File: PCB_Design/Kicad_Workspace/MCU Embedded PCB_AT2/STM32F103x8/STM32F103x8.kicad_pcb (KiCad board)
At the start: 2 copper layers, 68.8 x 61 mm, 16 parts, among them J1 Conn_01x17, J2 Conn_01x05, J3 Conn_01x01, J4 USB_A, J5 Conn_01x04, J6 Conn_01x08, SW1 SW_Push, U1 STM32F103C8Tx, U2 AP2204R-3.3, Y1 8MHz, Y2 32.768kHz

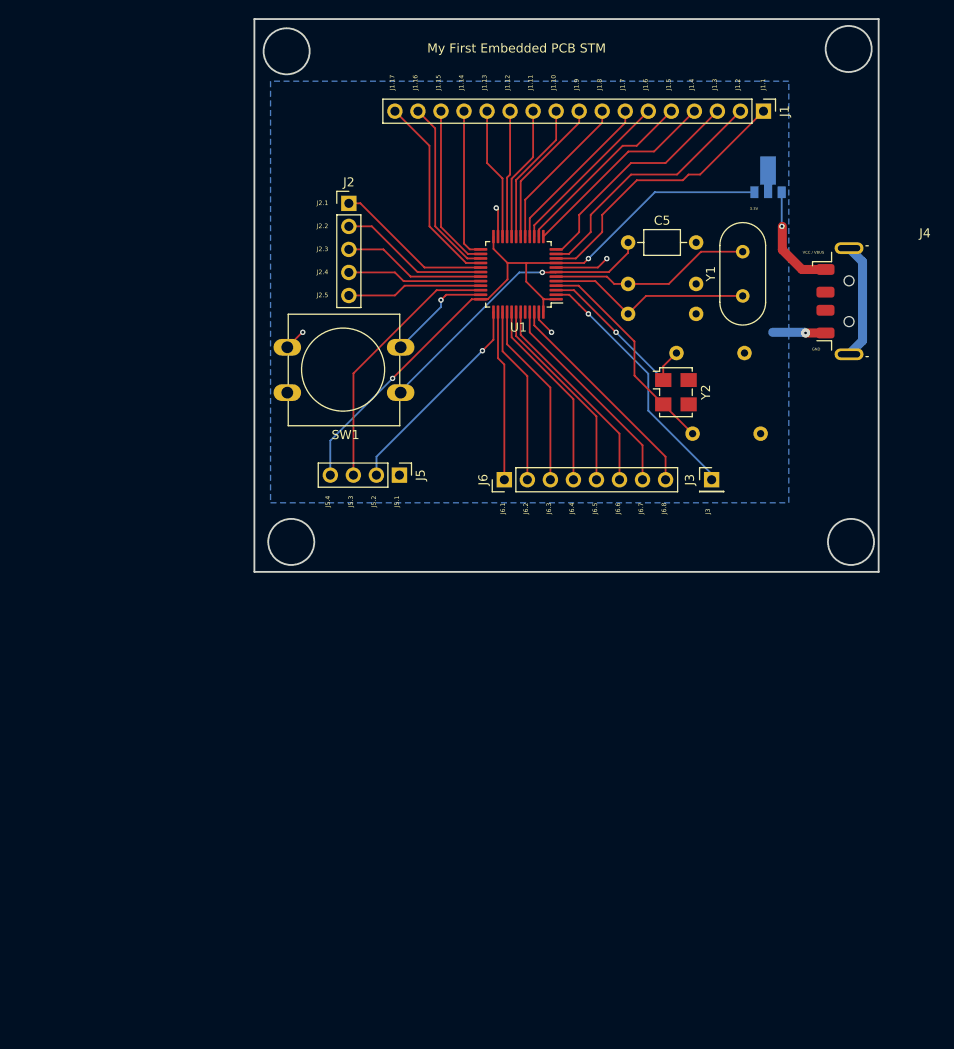
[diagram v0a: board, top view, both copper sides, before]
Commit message: update_stm
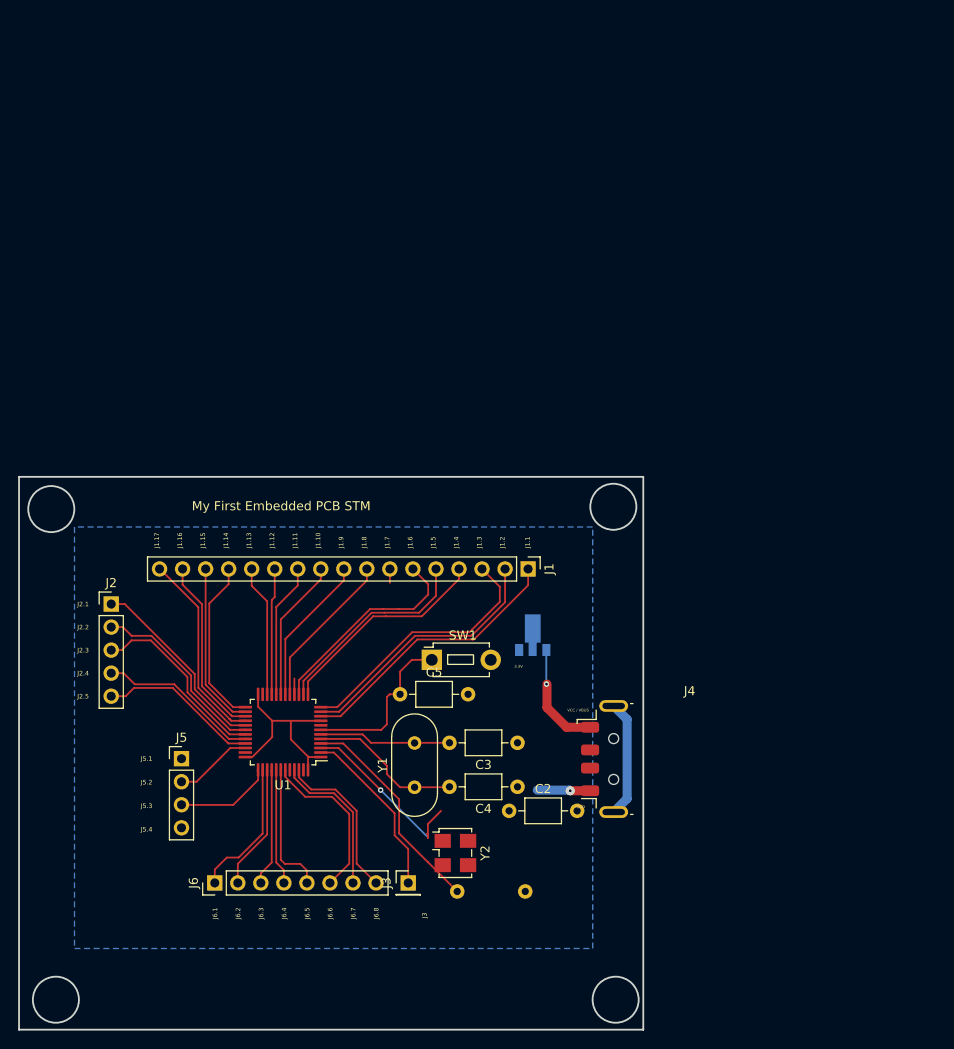
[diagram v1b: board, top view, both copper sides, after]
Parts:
- C2, C3, C4: moved to F.Cu
- SW1: footprint Button_Switch_THT:SW_PUSH-12mm -> Button_Switch_THT:SW_PUSH_1P1T_6x3.5mm_H4.3_APEM_MJTP1243
- moved Y1 65.2 mm to (134.2, 130.4)
- moved J4 56.8 mm to (164.6, 127.3)
- moved C2 56.8 mm to (144.7, 133.0), turned to 0 degrees
- moved J1 56.8 mm to (146.8, 106.4)
- moved U2 56.8 mm to (147.3, 113.3)
- moved C1 56.8 mm to (146.5, 141.9)
- moved U1 56.8 mm to (119.7, 124.3)
- moved Y2 56.3 mm to (138.7, 137.7)
- moved C5 55.8 mm to (132.6, 120.2)
- moved C4 55.7 mm to (145.6, 130.4)
- moved J3 55.6 mm to (133.5, 141.0)
- moved J6 54.7 mm to (112.2, 141.0)
- moved C3 54.3 mm to (145.6, 125.5)
- moved J2 51.4 mm to (100.8, 110.2)
- moved J5 39.4 mm to (108.5, 127.3), turned to 0 degrees
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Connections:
- J4 pad 5: unconnected-(J4-Shield-Pad5) -> GND
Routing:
- net +3V3: track 74.5 -> 22.2 mm, vias 2 -> 0
- net Net-(J5-Pin_2): track 29.0 -> 8.58 mm
- net Net-(J1-Pin_7): track 18.2 -> 3.30 mm
- net GND: track 33.2 -> 18.8 mm, vias 6 -> 1
- net Net-(U1-NRST): track 32.8 -> 18.7 mm, vias 1 -> 0
- net unconnected-(J4-Shield-Pad5): track 12.9 -> 0.00 mm
- net Net-(J5-Pin_3): track 23.4 -> 10.8 mm, vias 1 -> 0
- net Net-(J3-Pin_1): track 28.3 -> 19.2 mm, vias 1 -> 0
- net Net-(J6-Pin_4): track 21.3 -> 12.8 mm
- net Net-(U1-PD1-OSC_OUT): track 22.4 -> 14.5 mm
- net Net-(J6-Pin_5): track 22.2 -> 14.7 mm
- net Net-(J6-Pin_3): track 20.5 -> 13.0 mm
- net Net-(J6-Pin_7): track 23.6 -> 16.7 mm
- net Net-(J6-Pin_8): track 24.5 -> 17.6 mm
- net Net-(J6-Pin_2): track 19.6 -> 13.8 mm
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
